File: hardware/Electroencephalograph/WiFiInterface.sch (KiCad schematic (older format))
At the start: 20 parts, among them J7 Conn_01x04_Female, Q1 FDV304P, Q2 FDV304P, U12 ESP-12E

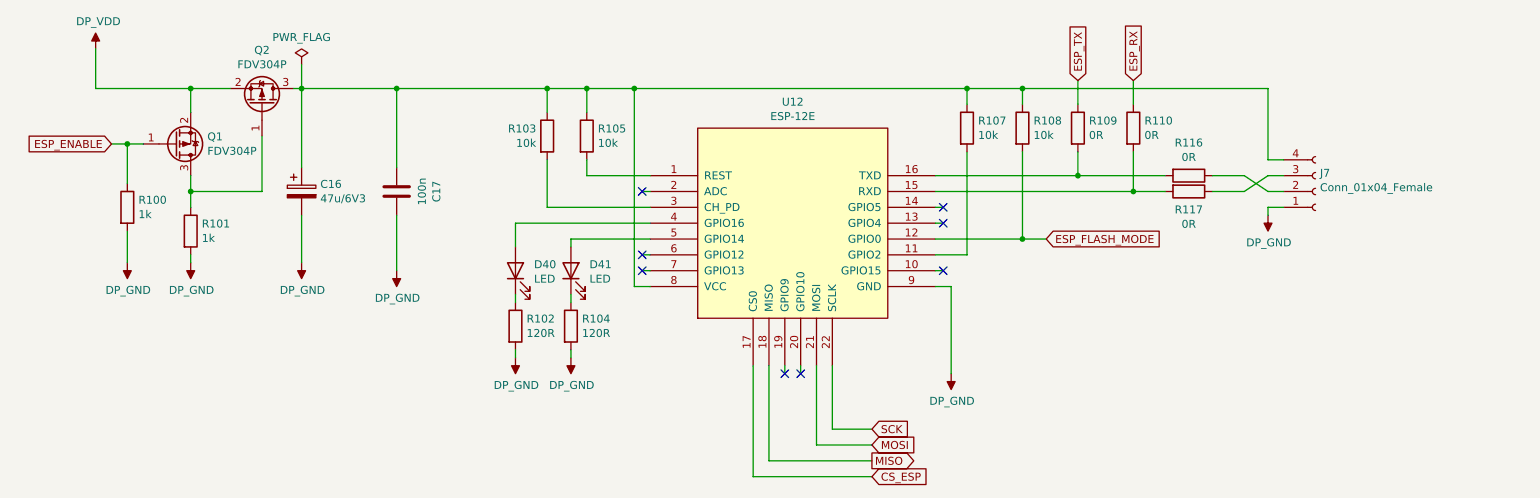
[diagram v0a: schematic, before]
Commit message: further routing of mcu part
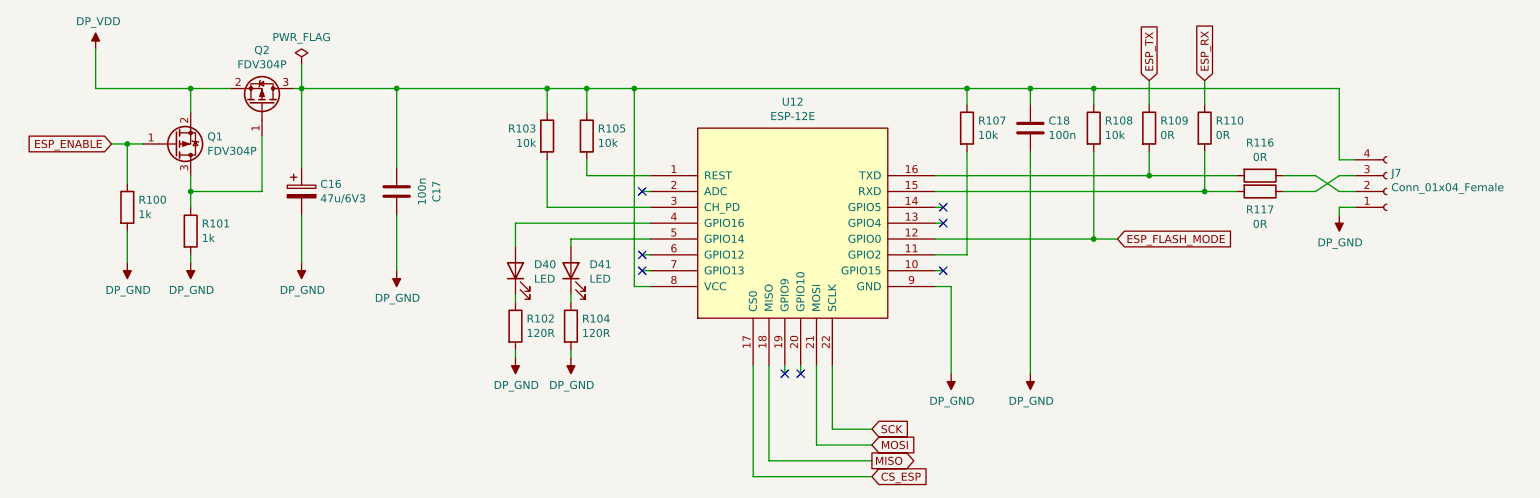
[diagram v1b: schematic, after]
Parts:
- added C18: 100n, Capacitor_SMD:C_0402_1005Metric, symbol Device:C
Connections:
- net DP_GND: now also C18.2
- net at C16.1, C17.1, J7.4 (Pin_4)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: now also C18.1
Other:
- moved on the sheet: J7, R108, R109, R110, R116, R117
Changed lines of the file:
@@
 L Connector:Conn_01x04_Female J?
 U 1 1 5F02C9FE
-P 9750 3350
+P 10200 3350
 AR Path="/5E142744/5F02C9FE" Ref="J?"  Part="1"
 AR Path="/5E27E78E/5F02C9FE" Ref="J?"  Part="1"
 AR Path="/5F01FBEA/5F02C9FE" Ref="J7"  Part="1"
-F 0 "J7" H 9778 3234 50  0000 L CNN
-F 1 "Conn_01x04_Female" H 9778 3325 50  0000 L CNN
-F 2 "Connector_PinHeader_2.54mm:PinHeader_1x04_P2.54mm_Vertical" H 9750 3350 50  0001 C CNN
-F 3 "~" H 9750 3350 50  0001 C CNN
-	1    9750 3350
+F 0 "J7" H 10228 3234 50  0000 L CNN
+F 1 "Conn_01x04_Female" H 10228 3325 50  0000 L CNN
+F 2 "Connector_PinHeader_2.54mm:PinHeader_1x04_P2.54mm_Vertical" H 10200 3350 50  0001 C CNN
+F 3 "~" H 10200 3350 50  0001 C CNN
+	1    10200 3350
 	1    0    0    1
 $EndComp
@@
 L Electroencephalograph:DP_GND #PWR?
 U 1 1 5F02CA04
-P 9450 3500
+P 9900 3500
 AR Path="/5F02CA04" Ref="#PWR?"  Part="1"
 AR Path="/5DAEEEF4/5F02CA04" Ref="#PWR?"  Part="1"
@@
 AR Path="/5E27E78E/5F02CA04" Ref="#PWR?"  Part="1"
 AR Path="/5F01FBEA/5F02CA04" Ref="#PWR231"  Part="1"
-F 0 "#PWR231" H 9450 3250 50  0001 C CNN
-F 1 "DP_GND" H 9455 3327 50  0000 C CNN
-F 2 "" H 9450 3500 50  0001 C CNN
-F 3 "" H 9450 3500 50  0001 C CNN
-	1    9450 3500
-	1    0    0    -1
-$EndComp
-Wire Wire Line
-	9550 3150 9450 3150
-Wire Wire Line
-	9450 3450 9450 3500
-Wire Wire Line
-	9550 3450 9450 3450
+F 0 "#PWR231" H 9900 3250 50  0001 C CNN
+F 1 "DP_GND" H 9905 3327 50  0000 C CNN
+F 2 "" H 9900 3500 50  0001 C CNN
+F 3 "" H 9900 3500 50  0001 C CNN
+	1    9900 3500
+	1    0    0    -1
+$EndComp
+Wire Wire Line
+	10000 3150 9900 3150
+Wire Wire Line
+	9900 3450 9900 3500
+Wire Wire Line
+	10000 3450 9900 3450
 Wire Wire Line
 	4900 2700 4900 2850
@@
 L Device:R R?
 U 1 1 5F02CA80
-P 7900 2950
+P 8350 2950
 AR Path="/5DD5C7F6/5F02CA80" Ref="R?"  Part="1"
 AR Path="/5DD5CD1D/5F02CA80" Ref="R?"  Part="1"
 AR Path="/5E27E78E/5F02CA80" Ref="R?"  Part="1"
 AR Path="/5F01FBEA/5F02CA80" Ref="R108"  Part="1"
-F 0 "R108" H 7970 2996 50  0000 L CNN
-F 1 "10k" H 7970 2905 50  0000 L CNN
-F 2 "Resistor_SMD:R_0402_1005Metric" V 7830 2950 50  0001 C CNN
-F 3 "~" H 7900 2950 50  0001 C CNN
-	1    7900 2950
-	1    0    0    -1
-$EndComp
-Text GLabel 8050 3650 2    50   Input ~ 0
+F 0 "R108" H 8420 2996 50  0000 L CNN
+F 1 "10k" H 8420 2905 50  0000 L CNN
+F 2 "Resistor_SMD:R_0402_1005Metric" V 8280 2950 50  0001 C CNN
+F 3 "~" H 8350 2950 50  0001 C CNN
+	1    8350 2950
+	1    0    0    -1
+$EndComp
+Text GLabel 8500 3650 2    50   Input ~ 0
 ESP_FLASH_MODE
 Wire Wire Line
-	9300 3350 9450 3250
-Wire Wire Line
-	9450 3350 9300 3250
-Wire Wire Line
-	9450 3250 9550 3250
-Wire Wire Line
-	9450 3350 9550 3350
-Wire Wire Line
-	8600 3350 8600 3100
-Wire Wire Line
-	8600 3350 8800 3350
-Text GLabel 8250 2650 1    50   Input ~ 0
+	9750 3350 9900 3250
+Wire Wire Line
+	9900 3350 9750 3250
+Wire Wire Line
+	9900 3250 10000 3250
+Wire Wire Line
+	9900 3350 10000 3350
+Wire Wire Line
+	9050 3350 9050 3100
+Wire Wire Line
+	9050 3350 9250 3350
+Text GLabel 8700 2650 1    50   Input ~ 0
 ESP_TX
-Text GLabel 8600 2650 1    50   Input ~ 0
+Text GLabel 9050 2650 1    50   Input ~ 0
 ESP_RX
 Wire Wire Line
-	7350 3350 8600 3350
-Connection ~ 8600 3350
+	7350 3350 9050 3350
+Connection ~ 9050 3350
 $Comp
 L Device:LED D?
@@
 L Device:R R?
 U 1 1 5F04FD04
-P 8250 2950
+P 8700 2950
 AR Path="/5DD5C7F6/5F04FD04" Ref="R?"  Part="1"
 AR Path="/5DD5CD1D/5F04FD04" Ref="R?"  Part="1"
 AR Path="/5E27E78E/5F04FD04" Ref="R?"  Part="1"
 AR Path="/5F01FBEA/5F04FD04" Ref="R109"  Part="1"
-F 0 "R109" H 8320 2996 50  0000 L CNN
-F 1 "0R" H 8320 2905 50  0000 L CNN
-F 2 "Resistor_SMD:R_0402_1005Metric" V 8180 2950 50  0001 C CNN
-F 3 "~" H 8250 2950 50  0001 C CNN
-	1    8250 2950
-	1    0    0    -1
-$EndComp
-Wire Wire Line
-	7350 3250 8250 3250
-Wire Wire Line
-	8250 2800 8250 2650
-Wire Wire Line
-	8250 3100 8250 3250
-Connection ~ 8250 3250
-Wire Wire Line
-	8250 3250 8800 3250
+F 0 "R109" H 8770 2996 50  0000 L CNN
+F 1 "0R" H 8770 2905 50  0000 L CNN
+F 2 "Resistor_SMD:R_0402_1005Metric" V 8630 2950 50  0001 C CNN
+F 3 "~" H 8700 2950 50  0001 C CNN
+	1    8700 2950
+	1    0    0    -1
+$EndComp
+Wire Wire Line
+	7350 3250 8700 3250
+Wire Wire Line
+	8700 2800 8700 2650
+Wire Wire Line
+	8700 3100 8700 3250
+Connection ~ 8700 3250
+Wire Wire Line
+	8700 3250 9250 3250
 $Comp
 L Device:R R?
 U 1 1 5F054862
-P 8600 2950
+P 9050 2950
 AR Path="/5DD5C7F6/5F054862" Ref="R?"  Part="1"
 AR Path="/5DD5CD1D/5F054862" Ref="R?"  Part="1"
 AR Path="/5E27E78E/5F054862" Ref="R?"  Part="1"
 AR Path="/5F01FBEA/5F054862" Ref="R110"  Part="1"
-F 0 "R110" H 8670 2996 50  0000 L CNN
-F 1 "0R" H 8670 2905 50  0000 L CNN
-F 2 "Resistor_SMD:R_0402_1005Metric" V 8530 2950 50  0001 C CNN
-F 3 "~" H 8600 2950 50  0001 C CNN
-	1    8600 2950
-	1    0    0    -1
-$EndComp
-Wire Wire Line
-	8600 2800 8600 2650
+F 0 "R110" H 9120 2996 50  0000 L CNN
+F 1 "0R" H 9120 2905 50  0000 L CNN
+F 2 "Resistor_SMD:R_0402_1005Metric" V 8980 2950 50  0001 C CNN
+F 3 "~" H 9050 2950 50  0001 C CNN
+	1    9050 2950
+	1    0    0    -1
+$EndComp
+Wire Wire Line
+	9050 2800 9050 2650
 Text GLabel 6950 4850 2    50   Input ~ 0
 SCK
@@
 L Device:R R?
 U 1 1 5F160F1A
-P 8950 3250
+P 9400 3250
 AR Path="/5DD5C7F6/5F160F1A" Ref="R?"  Part="1"
 AR Path="/5DD5CD1D/5F160F1A" Ref="R?"  Part="1"
 AR Path="/5E27E78E/5F160F1A" Ref="R?"  Part="1"
 AR Path="/5F01FBEA/5F160F1A" Ref="R116"  Part="1"
-F 0 "R116" V 8743 3250 50  0000 C CNN
-F 1 "0R" V 8834 3250 50  0000 C CNN
-F 2 "Resistor_SMD:R_0402_1005Metric" V 8880 3250 50  0001 C CNN
-F 3 "~" H 8950 3250 50  0001 C CNN
-	1    8950 3250
+F 0 "R116" V 9193 3250 50  0000 C CNN
+F 1 "0R" V 9284 3250 50  0000 C CNN
+F 2 "Resistor_SMD:R_0402_1005Metric" V 9330 3250 50  0001 C CNN
+F 3 "~" H 9400 3250 50  0001 C CNN
+	1    9400 3250
 	0    1    1    0
 $EndComp
 Wire Wire Line
-	9100 3250 9300 3250
+	9550 3250 9750 3250
 $Comp
 L Device:R R?
 U 1 1 5F161272
-P 8950 3350
+P 9400 3350
 AR Path="/5DD5C7F6/5F161272" Ref="R?"  Part="1"
 AR Path="/5DD5CD1D/5F161272" Ref="R?"  Part="1"
 AR Path="/5E27E78E/5F161272" Ref="R?"  Part="1"
 AR Path="/5F01FBEA/5F161272" Ref="R117"  Part="1"
-F 0 "R117" V 9065 3350 50  0000 C CNN
-F 1 "0R" V 9156 3350 50  0000 C CNN
-F 2 "Resistor_SMD:R_0402_1005Metric" V 8880 3350 50  0001 C CNN
-F 3 "~" H 8950 3350 50  0001 C CNN
-	1    8950 3350
+F 0 "R117" V 9515 3350 50  0000 C CNN
+F 1 "0R" V 9606 3350 50  0000 C CNN
+F 2 "Resistor_SMD:R_0402_1005Metric" V 9330 3350 50  0001 C CNN
+F 3 "~" H 9400 3350 50  0001 C CNN
+	1    9400 3350
 	0    1    1    0
 $EndComp
 Wire Wire Line
-	9100 3350 9300 3350
+	9550 3350 9750 3350
 Wire Wire Line
 	5450 2700 7550 2700
 Wire Wire Line
-	7550 2700 7900 2700
-Wire Wire Line
-	7900 2700 7900 2800
+	7550 2700 7950 2700
+Wire Wire Line
+	8350 2700 8350 2800
 Connection ~ 7550 2700
 Wire Wire Line
-	7900 3100 7900 3650
-Wire Wire Line
-	7350 3650 7900 3650
-Connection ~ 7900 3650
-Wire Wire Line
-	7900 3650 8050 3650
-Wire Wire Line
-	7900 2700 9450 2700
-Wire Wire Line
-	9450 2700 9450 3150
-Connection ~ 7900 2700
+	8350 3100 8350 3650
+Wire Wire Line
+	7350 3650 8350 3650
+Connection ~ 8350 3650
+Wire Wire Line
+	8350 3650 8500 3650
+Wire Wire Line
+	8350 2700 9900 2700
+Wire Wire Line
+	9900 2700 9900 3150
+Connection ~ 8350 2700
+$Comp
+L Device:C C?
+U 1 1 5F0FAD1C
+P 7950 2950
+AR Path="/5F0FAD1C" Ref="C?"  Part="1"
+AR Path="/5DAEEEF4/5F0FAD1C" Ref="C?"  Part="1"
+AR Path="/5DD5C7F6/5F0FAD1C" Ref="C?"  Part="1"
+AR Path="/5DD5CD1D/5F0FAD1C" Ref="C?"  Part="1"
+AR Path="/5E27E78E/5F0FAD1C" Ref="C?"  Part="1"
+AR Path="/5F01FBEA/5F0FAD1C" Ref="C18"  Part="1"
+F 0 "C18" H 8065 2996 50  0000 L CNN
+F 1 "100n" H 8065 2905 50  0000 L CNN
+F 2 "Capacitor_SMD:C_0402_1005Metric" H 7988 2800 50  0001 C CNN
+F 3 "~" H 7950 2950 50  0001 C CNN
+	1    7950 2950
+	1    0    0    -1
+$EndComp
+$Comp
+L Electroencephalograph:DP_GND #PWR?
+U 1 1 5F0FB11C
+P 7950 4500
+AR Path="/5F0FB11C" Ref="#PWR?"  Part="1"
+AR Path="/5DAEEEF4/5F0FB11C" Ref="#PWR?"  Part="1"
+AR Path="/5DD5C7F6/5F0FB11C" Ref="#PWR?"  Part="1"
+AR Path="/5DD5CD1D/5F0FB11C" Ref="#PWR?"  Part="1"
+AR Path="/5E27E78E/5F0FB11C" Ref="#PWR?"  Part="1"
+AR Path="/5F01FBEA/5F0FB11C" Ref="#PWR228"  Part="1"
+F 0 "#PWR228" H 7950 4250 50  0001 C CNN
+F 1 "DP_GND" H 7955 4327 50  0000 C CNN
+F 2 "" H 7950 4500 50  0001 C CNN
+F 3 "" H 7950 4500 50  0001 C CNN
+	1    7950 4500
+	1    0    0    -1
+$EndComp
+Wire Wire Line
+	7950 4500 7950 3100
+Wire Wire Line
+	7950 2800 7950 2700
+Connection ~ 7950 2700
+Wire Wire Line
+	7950 2700 8350 2700
 $EndSCHEMATC
